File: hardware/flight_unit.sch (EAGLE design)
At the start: 26 parts, among them IC2 7805T, J2 CONN_20X2SHROUDED, T1 THERMISTOR-2,5, U1 4MB Flash, U2 4MB Flash, U3 4MB Flash

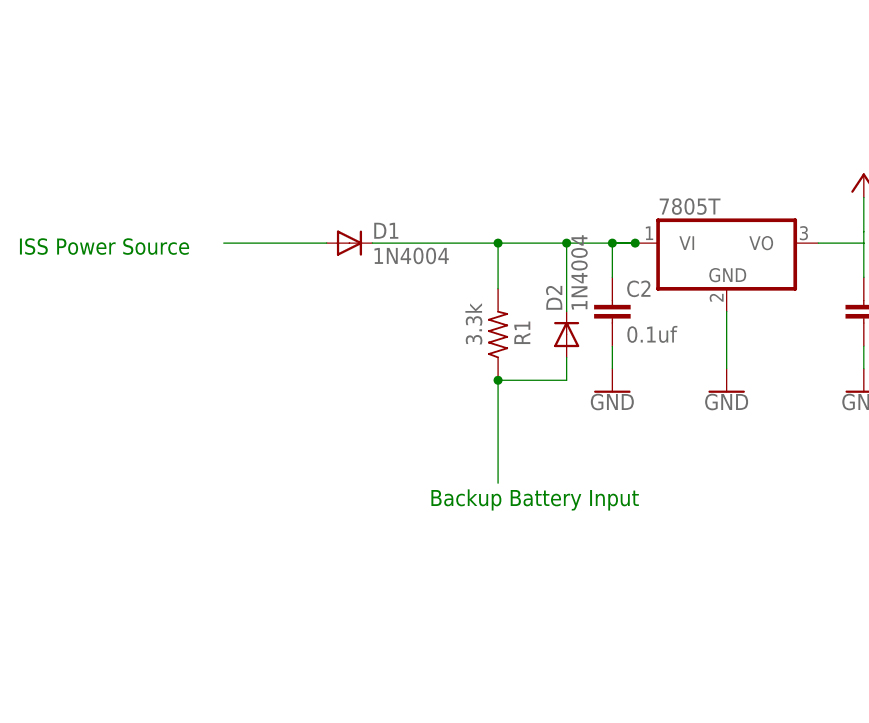
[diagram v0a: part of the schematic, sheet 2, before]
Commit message: Add files via upload
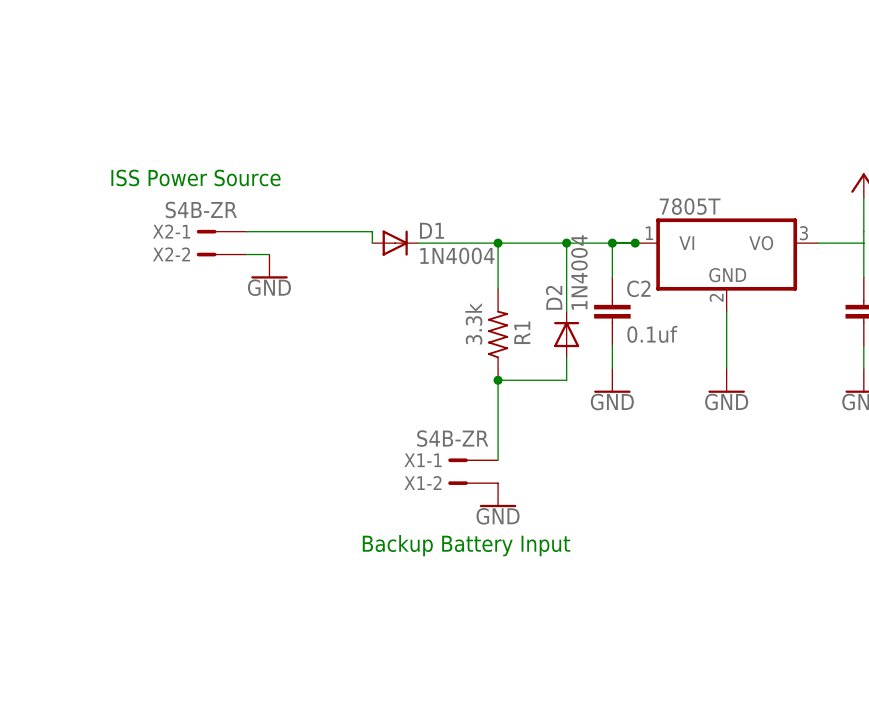
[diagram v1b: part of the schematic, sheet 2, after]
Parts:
- added X1, X2: S4B-ZR, con-jst:S4B-ZR
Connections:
- net GND: now also X1-2.1, X2-2.1
- net N$1: now also X1-1.1
- net N$4: now also X2-1.1
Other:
- moved on the sheet: D1
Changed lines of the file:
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@@
 <part name="C2" library="capacitor-wima" library_urn="urn:adsk.eagle:library:116" deviceset="C" device="2,5-3" package3d_urn="urn:adsk.eagle:package:5436/1" value="0.1uf"/>
 <part name="GND2" library="SparkFun-PowerSymbols" library_urn="urn:adsk.eagle:library:530" deviceset="GND" device=""/>
+<part name="X1" library="con-jst" library_urn="urn:adsk.eagle:library:156" deviceset="?4B-ZR" device="S" package3d_urn="urn:adsk.eagle:package:7641/1"/>
+<part name="X2" library="con-jst" library_urn="urn:adsk.eagle:library:156" deviceset="?4B-ZR" device="S" package3d_urn="urn:adsk.eagle:package:7641/1"/>
+<part name="GND9" library="SparkFun-PowerSymbols" library_urn="urn:adsk.eagle:library:530" deviceset="GND" device=""/>
+<part name="GND10" library="SparkFun-PowerSymbols" library_urn="urn:adsk.eagle:library:530" deviceset="GND" device=""/>
 </parts>
 <sheets>
@@
 </text>
 <text x="82.55" y="161.29" size="5.08" layer="97">Power Regulation and Supply</text>
-<text x="68.58" y="109.22" size="1.778" layer="91">ISS Power Source</text>
-<text x="114.3" y="81.28" size="1.778" layer="91">Backup Battery Input </text>
+<text x="78.74" y="116.84" size="1.778" layer="91">ISS Power Source</text>
+<text x="106.68" y="76.2" size="1.778" layer="91">Backup Battery Input </text>
 </plain>
 <instances>
@@
 <attribute name="SHEET" x="230.505" y="5.08" size="2.54" layer="94"/>
 </instance>
-<instance part="D1" gate="1" x="105.41" y="110.49" smashed="yes">
-<attribute name="NAME" x="107.95" y="110.9726" size="1.778" layer="95"/>
-<attribute name="VALUE" x="107.95" y="108.1786" size="1.778" layer="96"/>
+<instance part="D1" gate="1" x="110.49" y="110.49" smashed="yes">
+<attribute name="NAME" x="113.03" y="110.9726" size="1.778" layer="95"/>
+<attribute name="VALUE" x="113.03" y="108.1786" size="1.778" layer="96"/>
 </instance>
 <instance part="D2" gate="1" x="129.54" y="100.33" smashed="yes" rot="R90">
@@
 <instance part="GND2" gate="1" x="134.62" y="93.98" smashed="yes">
 <attribute name="VALUE" x="134.62" y="93.726" size="1.778" layer="96" align="top-center"/>
+</instance>
+<instance part="X1" gate="-1" x="116.84" y="86.36" smashed="yes" rot="MR0">
+<attribute name="NAME" x="115.824" y="85.598" size="1.524" layer="95" rot="MR0"/>
+<attribute name="VALUE" x="120.904" y="87.884" size="1.778" layer="96" rot="MR0"/>
+</instance>
+<instance part="X1" gate="-2" x="116.84" y="83.82" smashed="yes" rot="MR0">
+<attribute name="NAME" x="115.824" y="83.058" size="1.524" layer="95" rot="MR0"/>
+</instance>
+<instance part="X2" gate="-1" x="88.9" y="111.76" smashed="yes" rot="MR0">
+<attribute name="NAME" x="87.884" y="110.998" size="1.524" layer="95" rot="MR0"/>
+<attribute name="VALUE" x="92.964" y="113.284" size="1.778" layer="96" rot="MR0"/>
+</instance>
+<instance part="X2" gate="-2" x="88.9" y="109.22" smashed="yes" rot="MR0">
+<attribute name="NAME" x="87.884" y="108.458" size="1.524" layer="95" rot="MR0"/>
+</instance>
+<instance part="GND9" gate="1" x="96.52" y="106.68" smashed="yes">
+<attribute name="VALUE" x="96.52" y="106.426" size="1.778" layer="96" align="top-center"/>
+</instance>
+<instance part="GND10" gate="1" x="121.92" y="81.28" smashed="yes">
+<attribute name="VALUE" x="121.92" y="81.026" size="1.778" layer="96" align="top-center"/>
 </instance>
 </instances>
@@
 <wire x1="121.92" y1="95.25" x2="129.54" y2="95.25" width="0.1524" layer="91"/>
 <wire x1="129.54" y1="95.25" x2="129.54" y2="97.79" width="0.1524" layer="91"/>
-<wire x1="121.92" y1="95.25" x2="121.92" y2="83.82" width="0.1524" layer="91"/>
+<pinref part="X1" gate="-1" pin="1"/>
+<wire x1="121.92" y1="86.36" x2="121.92" y2="95.25" width="0.1524" layer="91"/>
 <junction x="121.92" y="95.25"/>
 </segment>
@@
 <pinref part="D1" gate="1" pin="C"/>
 <pinref part="R1" gate="G$1" pin="2"/>
-<wire x1="107.95" y1="110.49" x2="121.92" y2="110.49" width="0.1524" layer="91"/>
+<wire x1="113.03" y1="110.49" x2="121.92" y2="110.49" width="0.1524" layer="91"/>
 <wire x1="121.92" y1="110.49" x2="121.92" y2="105.41" width="0.1524" layer="91"/>
 <junction x="121.92" y="110.49"/>
@@
 </segment>
 </net>
-<net name="N$4" class="0">
-<segment>
-<pinref part="D1" gate="1" pin="A"/>
-<wire x1="91.44" y1="110.49" x2="102.87" y2="110.49" width="0.1524" layer="91"/>
-</segment>
-</net>
 <net name="+3V3" class="0">
 <segment>
@@
 <wire x1="134.62" y1="99.06" x2="134.62" y2="96.52" width="0.1524" layer="91"/>
 </segment>
+<segment>
+<pinref part="X2" gate="-2" pin="1"/>
+<pinref part="GND9" gate="1" pin="GND"/>
+<wire x1="93.98" y1="109.22" x2="96.52" y2="109.22" width="0.1524" layer="91"/>
+</segment>
+<segment>
+<pinref part="GND10" gate="1" pin="GND"/>
+<pinref part="X1" gate="-2" pin="1"/>
+</segment>
 </net>
 <net name="N$9" class="0">
@@
 </segment>
 </net>
+<net name="N$4" class="0">
+<segment>
+<pinref part="X2" gate="-1" pin="1"/>
+<pinref part="D1" gate="1" pin="A"/>
+<wire x1="93.98" y1="111.76" x2="107.95" y2="111.76" width="0.1524" layer="91"/>
+<wire x1="107.95" y1="111.76" x2="107.95" y2="110.49" width="0.1524" layer="91"/>
+</segment>
+</net>
